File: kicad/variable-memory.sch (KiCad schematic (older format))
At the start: 1 part

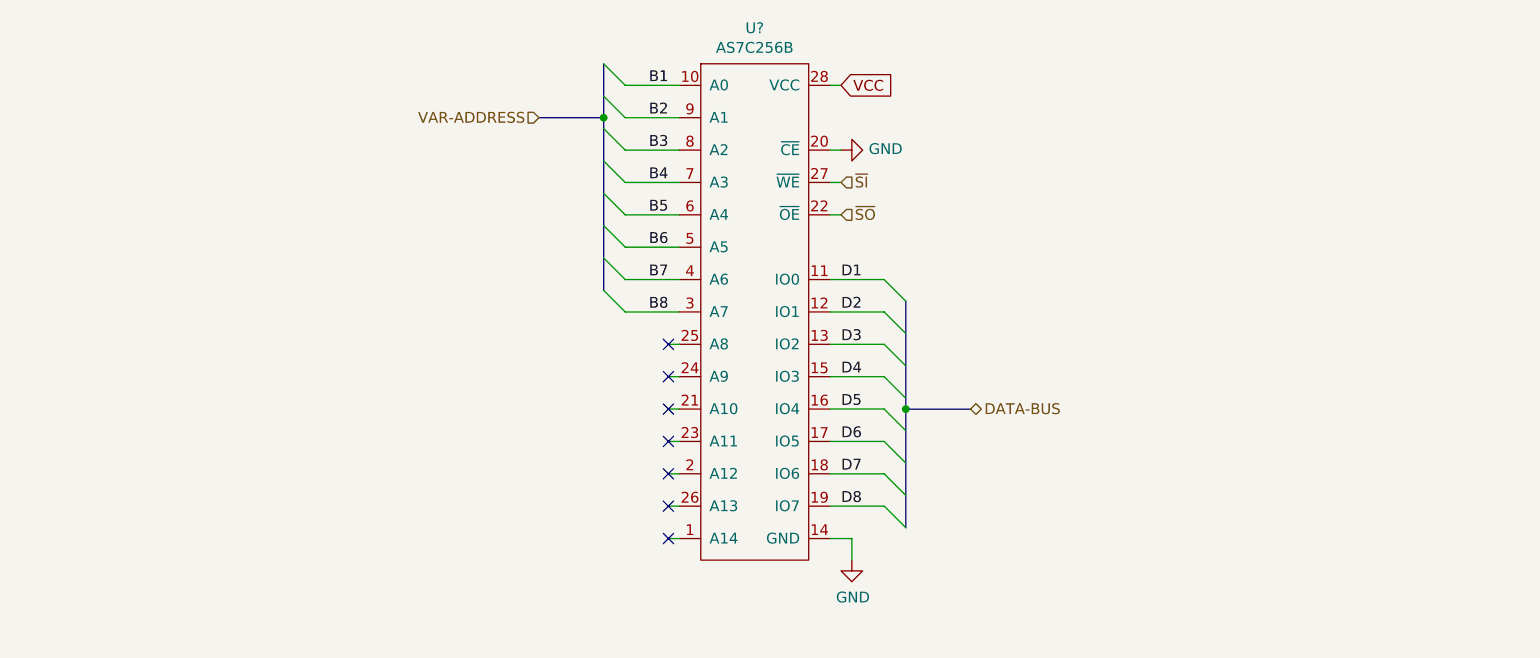
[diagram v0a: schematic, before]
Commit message: Final Commit Pre-Talk The final commit before Monday's talk, including the PDF of the schematic to make it accessible.
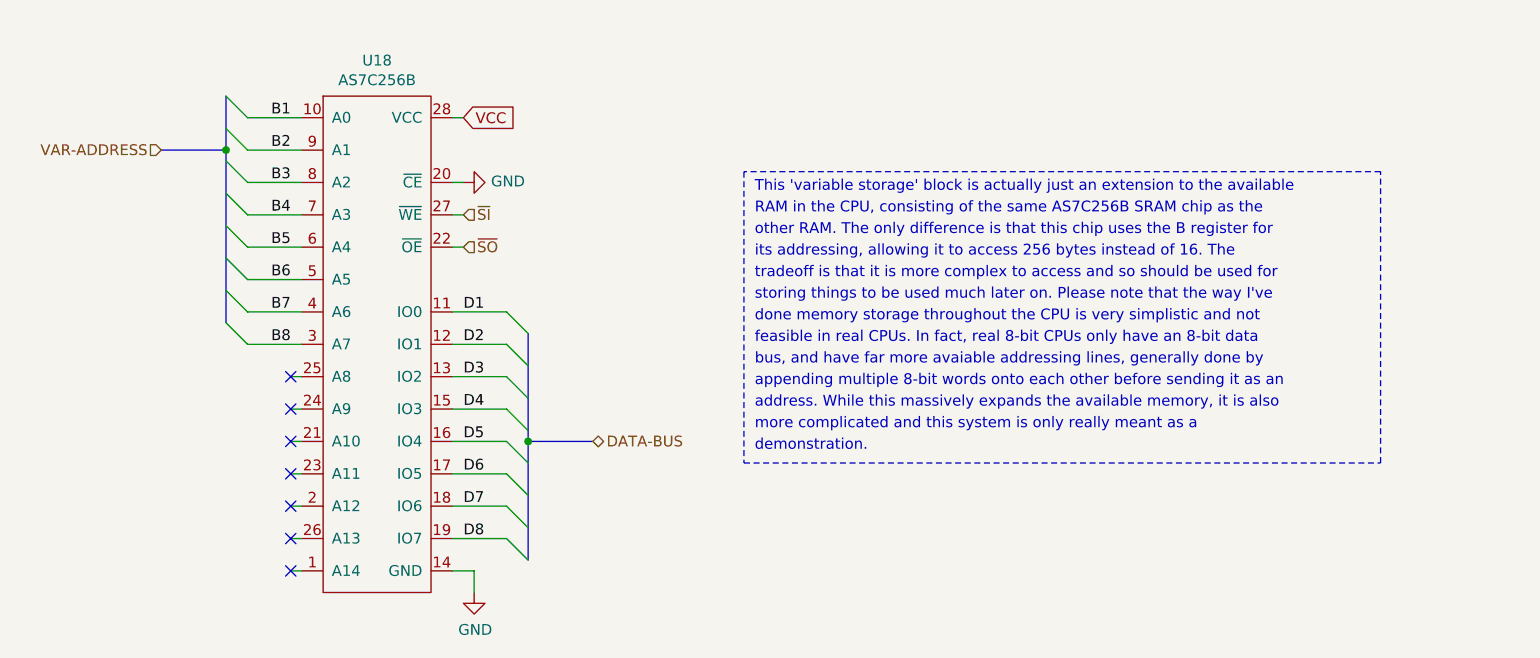
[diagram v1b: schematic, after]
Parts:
- gave numbers to parts that had none: 1
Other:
- note added: "RAM in the CPU, consisting of the same AS7C256B SRAM chip as the"
- note added: "This 'variable storage' block is actually just an extension to the available"
- note added: "address. While this massively expands the available memory, it is also"
- note added: "appending multiple 8-bit words onto each other before sending it as an"
- note added: "bus, and have far more avaiable addressing lines, generally done by"
- note added: "demonstration."
- note added: "done memory storage throughout the CPU is very simplistic and not"
- note added: "feasible in real CPUs. In fact, real 8-bit CPUs only have an 8-bit data"
- note added: "its addressing, allowing it to access 256 bytes instead of 16. The"
- note added: "more complicated and this system is only really meant as a"
- note added: "other RAM. The only difference is that this chip uses the B register for"
- note added: "storing things to be used much later on. Please note that the way I've"
- note added: "tradeoff is that it is more complex to access and so should be used for"
- moved on the sheet: U18
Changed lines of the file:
@@
 $Descr A4 11693 8268
 encoding utf-8
-Sheet 10 13
+Sheet 10 14
 Title "Variable Memory"
 Date "2019-11-11"
@@
 Comment4 "Author: Sebastian Gaume"
 $EndDescr
-Text HLabel 4900 2850 0    50   Input ~ 0
+Text HLabel 3150 3000 0    50   Input ~ 0
 VAR-ADDRESS
 Wire Wire Line
-	5550 2700 5300 2700
-Wire Wire Line
-	5300 2850 5550 2850
-Wire Wire Line
-	5550 3000 5300 3000
-Wire Wire Line
-	5300 3150 5550 3150
-Entry Wire Line
-	5200 3050 5300 3150
-Entry Wire Line
-	5200 2900 5300 3000
-Entry Wire Line
-	5200 2750 5300 2850
-Entry Wire Line
-	5200 2600 5300 2700
-Wire Wire Line
-	6250 3000 6300 3000
+	3800 2850 3550 2850
+Wire Wire Line
+	3550 3000 3800 3000
+Wire Wire Line
+	3800 3150 3550 3150
+Wire Wire Line
+	3550 3300 3800 3300
+Entry Wire Line
+	3450 3200 3550 3300
+Entry Wire Line
+	3450 3050 3550 3150
+Entry Wire Line
+	3450 2900 3550 3000
+Entry Wire Line
+	3450 2750 3550 2850
+Wire Wire Line
+	4500 3150 4550 3150
 $Comp
 L power:GND #PWR?
 U 1 1 5DDF34EA
-P 6300 3000
+P 4550 3150
 AR Path="/5DDC3596/5DDF34EA" Ref="#PWR?"  Part="1"
-AR Path="/5DDEF819/5DDF34EA" Ref="#PWR?"  Part="1"
-F 0 "#PWR?" H 6300 2750 50  0001 C CNN
-F 1 "GND" V 6305 2872 50  0000 R CNN
-F 2 "" H 6300 3000 50  0001 C CNN
-F 3 "" H 6300 3000 50  0001 C CNN
-	1    6300 3000
+AR Path="/5DDEF819/5DDF34EA" Ref="#PWR0127"  Part="1"
+F 0 "#PWR0127" H 4550 2900 50  0001 C CNN
+F 1 "GND" V 4555 3022 50  0000 R CNN
+F 2 "" H 4550 3150 50  0001 C CNN
+F 3 "" H 4550 3150 50  0001 C CNN
+	1    4550 3150
 	0    -1   -1   0
 $EndComp
 Wire Wire Line
-	6250 3150 6300 3150
-Wire Wire Line
-	6250 3300 6300 3300
-Text HLabel 6300 3150 2    50   Input ~ 0
+	4500 3300 4550 3300
+Wire Wire Line
+	4500 3450 4550 3450
+Text HLabel 4550 3300 2    50   Input ~ 0
 ~SI~
-Text HLabel 6300 3300 2    50   Input ~ 0
+Text HLabel 4550 3450 2    50   Input ~ 0
 ~SO~
 Wire Wire Line
-	5550 3900 5500 3900
-Wire Wire Line
-	5500 4050 5550 4050
-Wire Wire Line
-	5550 4200 5500 4200
-Wire Wire Line
-	5500 4350 5550 4350
-Wire Wire Line
-	5550 4500 5500 4500
-Wire Wire Line
-	5500 4650 5550 4650
-Wire Wire Line
-	5550 4800 5500 4800
-NoConn ~ 5500 3900
-NoConn ~ 5500 4050
-NoConn ~ 5500 4200
-NoConn ~ 5500 4350
-NoConn ~ 5500 4500
-NoConn ~ 5500 4650
-NoConn ~ 5500 4800
-Wire Bus Line
-	4900 2850 5200 2850
-Connection ~ 5200 2850
-Wire Wire Line
-	6250 2700 6300 2700
-Text GLabel 6300 2700 2    50   Input ~ 0
+	3800 4050 3750 4050
+Wire Wire Line
+	3750 4200 3800 4200
+Wire Wire Line
+	3800 4350 3750 4350
+Wire Wire Line
+	3750 4500 3800 4500
+Wire Wire Line
+	3800 4650 3750 4650
+Wire Wire Line
+	3750 4800 3800 4800
+Wire Wire Line
+	3800 4950 3750 4950
+NoConn ~ 3750 4050
+NoConn ~ 3750 4200
+NoConn ~ 3750 4350
+NoConn ~ 3750 4500
+NoConn ~ 3750 4650
+NoConn ~ 3750 4800
+NoConn ~ 3750 4950
+Wire Bus Line
+	3150 3000 3450 3000
+Connection ~ 3450 3000
+Wire Wire Line
+	4500 2850 4550 2850
+Text GLabel 4550 2850 2    50   Input ~ 0
 VCC
 Wire Wire Line
-	6250 4800 6350 4800
-Wire Wire Line
-	6350 4800 6350 4900
+	4500 4950 4600 4950
+Wire Wire Line
+	4600 4950 4600 5050
 $Comp
 L power:GND #PWR?
 U 1 1 5DDF3510
-P 6350 4900
+P 4600 5050
 AR Path="/5DDC3596/5DDF3510" Ref="#PWR?"  Part="1"
-AR Path="/5DDEF819/5DDF3510" Ref="#PWR?"  Part="1"
-F 0 "#PWR?" H 6350 4650 50  0001 C CNN
-F 1 "GND" H 6355 4727 50  0000 C CNN
-F 2 "" H 6350 4900 50  0001 C CNN
-F 3 "" H 6350 4900 50  0001 C CNN
-	1    6350 4900
+AR Path="/5DDEF819/5DDF3510" Ref="#PWR0128"  Part="1"
+F 0 "#PWR0128" H 4600 4800 50  0001 C CNN
+F 1 "GND" H 4605 4877 50  0000 C CNN
+F 2 "" H 4600 5050 50  0001 C CNN
+F 3 "" H 4600 5050 50  0001 C CNN
+	1    4600 5050
 	1    0    0    -1
 $EndComp
 Wire Wire Line
-	6250 3600 6500 3600
-Wire Wire Line
-	6500 3750 6250 3750
-Wire Wire Line
-	6250 3900 6500 3900
-Wire Wire Line
-	6500 4050 6250 4050
-Wire Wire Line
-	6250 4200 6500 4200
-Wire Wire Line
-	6500 4350 6250 4350
-Wire Wire Line
-	6250 4500 6500 4500
-Wire Wire Line
-	6500 4650 6250 4650
-Entry Wire Line
-	6500 3600 6600 3700
-Entry Wire Line
-	6500 3750 6600 3850
-Entry Wire Line
-	6500 3900 6600 4000
-Entry Wire Line
-	6500 4050 6600 4150
-Entry Wire Line
-	6500 4200 6600 4300
-Entry Wire Line
-	6500 4350 6600 4450
-Entry Wire Line
-	6500 4500 6600 4600
-Entry Wire Line
-	6500 4650 6600 4750
-Wire Bus Line
-	6600 4200 6900 4200
-Connection ~ 6600 4200
-Text HLabel 6900 4200 2    50   BiDi ~ 0
+	4500 3750 4750 3750
+Wire Wire Line
+	4750 3900 4500 3900
+Wire Wire Line
+	4500 4050 4750 4050
+Wire Wire Line
+	4750 4200 4500 4200
+Wire Wire Line
+	4500 4350 4750 4350
+Wire Wire Line
+	4750 4500 4500 4500
+Wire Wire Line
+	4500 4650 4750 4650
+Wire Wire Line
+	4750 4800 4500 4800
+Entry Wire Line
+	4750 3750 4850 3850
+Entry Wire Line
+	4750 3900 4850 4000
+Entry Wire Line
+	4750 4050 4850 4150
+Entry Wire Line
+	4750 4200 4850 4300
+Entry Wire Line
+	4750 4350 4850 4450
+Entry Wire Line
+	4750 4500 4850 4600
+Entry Wire Line
+	4750 4650 4850 4750
+Entry Wire Line
+	4750 4800 4850 4900
+Wire Bus Line
+	4850 4350 5150 4350
+Connection ~ 4850 4350
+Text HLabel 5150 4350 2    50   BiDi ~ 0
 DATA-BUS
-Text Label 6300 3600 0    50   ~ 0
+Text Label 4550 3750 0    50   ~ 0
 D1
-Text Label 6300 3750 0    50   ~ 0
+Text Label 4550 3900 0    50   ~ 0
 D2
-Text Label 6300 3900 0    50   ~ 0
+Text Label 4550 4050 0    50   ~ 0
 D3
-Text Label 6300 4050 0    50   ~ 0
+Text Label 4550 4200 0    50   ~ 0
 D4
-Text Label 6300 4200 0    50   ~ 0
+Text Label 4550 4350 0    50   ~ 0
 D5
-Text Label 6300 4350 0    50   ~ 0
+Text Label 4550 4500 0    50   ~ 0
 D6
-Text Label 6300 4500 0    50   ~ 0
+Text Label 4550 4650 0    50   ~ 0
 D7
-Text Label 6300 4650 0    50   ~ 0
+Text Label 4550 4800 0    50   ~ 0
 D8
 $Comp
 L 8-bit-computer-other:AS7C256B U?
 U 1 1 5DDF3516
-P 5900 3750
+P 4150 3900
 AR Path="/5DDC3596/5DDF3516" Ref="U?"  Part="1"
-AR Path="/5DDEF819/5DDF3516" Ref="U?"  Part="1"
-F 0 "U?" H 5900 5065 50  0000 C CNN
-F 1 "AS7C256B" H 5900 4974 50  0000 C CNN
-F 2 "" V 5900 3700 50  0001 C CNN
-F 3 "" V 5900 3700 50  0001 C CNN
-	1    5900 3750
+AR Path="/5DDEF819/5DDF3516" Ref="U18"  Part="1"
+F 0 "U18" H 4150 5215 50  0000 C CNN
+F 1 "AS7C256B" H 4150 5124 50  0000 C CNN
+F 2 "" V 4150 3850 50  0001 C CNN
+F 3 "" V 4150 3850 50  0001 C CNN
+	1    4150 3900
 	1    0    0    -1
 $EndComp
 Wire Wire Line
-	5550 3300 5300 3300
-Wire Wire Line
-	5300 3450 5550 3450
-Wire Wire Line
-	5550 3600 5300 3600
-Wire Wire Line
-	5300 3750 5550 3750
-Entry Wire Line
-	5200 3200 5300 3300
-Entry Wire Line
-	5200 3350 5300 3450
-Entry Wire Line
-	5200 3500 5300 3600
-Entry Wire Line
-	5200 3650 5300 3750
-Text Label 5500 2700 2    50   ~ 0
+	3800 3450 3550 3450
+Wire Wire Line
+	3550 3600 3800 3600
+Wire Wire Line
+	3800 3750 3550 3750
+Wire Wire Line
+	3550 3900 3800 3900
+Entry Wire Line
+	3450 3350 3550 3450
+Entry Wire Line
+	3450 3500 3550 3600
+Entry Wire Line
+	3450 3650 3550 3750
+Entry Wire Line
+	3450 3800 3550 3900
+Text Label 3750 2850 2    50   ~ 0
 B1
-Text Label 5500 2850 2    50   ~ 0
+Text Label 3750 3000 2    50   ~ 0
 B2
-Text Label 5500 3000 2    50   ~ 0
+Text Label 3750 3150 2    50   ~ 0
 B3
-Text Label 5500 3150 2    50   ~ 0
+Text Label 3750 3300 2    50   ~ 0
 B4
-Text Label 5500 3300 2    50   ~ 0
+Text Label 3750 3450 2    50   ~ 0
 B5
-Text Label 5500 3450 2    50   ~ 0
+Text Label 3750 3600 2    50   ~ 0
 B6
-Text Label 5500 3600 2    50   ~ 0
+Text Label 3750 3750 2    50   ~ 0
 B7
-Text Label 5500 3750 2    50   ~ 0
+Text Label 3750 3900 2    50   ~ 0
 B8
-Wire Bus Line
-	5200 2600 5200 2850
-Wire Bus Line
-	6600 4200 6600 4750
-Wire Bus Line
-	6600 3700 6600 4200
-Wire Bus Line
-	5200 2850 5200 3650
+Text Notes 5900 3200 0    50   ~ 0
+This 'variable storage' block is actually just an extension to the available
+Text Notes 5900 3300 0    50   ~ 0
+RAM in the CPU, consisting of the same AS7C256B SRAM chip as the
+Text Notes 5900 3400 0    50   ~ 0
+other RAM. The only difference is that this chip uses the B register for
+Text Notes 5900 3500 0    50   ~ 0
+its addressing, allowing it to access 256 bytes instead of 16. The
+Text Notes 5900 3600 0    50   ~ 0
+tradeoff is that it is more complex to access and so should be used for
+Text Notes 5900 3700 0    50   ~ 0
+storing things to be used much later on. Please note that the way I've
+Text Notes 5900 3800 0    50   ~ 0
+done memory storage throughout the CPU is very simplistic and not
+Text Notes 5900 3900 0    50   ~ 0
+feasible in real CPUs. In fact, real 8-bit CPUs only have an 8-bit data
+Text Notes 5900 4000 0    50   ~ 0
+bus, and have far more avaiable addressing lines, generally done by
+Text Notes 5900 4100 0    50   ~ 0
+appending multiple 8-bit words onto each other before sending it as an
+Text Notes 5900 4200 0    50   ~ 0
+address. While this massively expands the available memory, it is also
+Text Notes 5900 4300 0    50   ~ 0
+more complicated and this system is only really meant as a
+Text Notes 5900 4400 0    50   ~ 0
+demonstration.
+Wire Notes Line
+	5850 3100 5850 4450
+Wire Notes Line
+	5850 4450 8800 4450
+Wire Notes Line
+	8800 4450 8800 3100
+Wire Notes Line
+	8800 3100 5850 3100
+Wire Bus Line
+	3450 2750 3450 3000
+Wire Bus Line
+	4850 4350 4850 4900
+Wire Bus Line
+	4850 3850 4850 4350
+Wire Bus Line
+	3450 3000 3450 3800
 $EndSCHEMATC
